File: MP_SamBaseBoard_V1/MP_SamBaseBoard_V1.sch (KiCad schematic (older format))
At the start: 126 parts, among them J1 MA_CONN, J10 P1_CONN, J11 I2C_CONN, J12 I2C_CONN, J13 SAM_SWD, J14 WS2812_EXT, J15 PWR_JACK, J16 USB_B_Micro, J17 BATT_CONN, J2 MB_CONN, J3 Adafruit_Feather_CONN, J4 LOAD_CONN, J5 SPEAKER, J7 SERVO_CONN, J8 P3_CONN, J9 P2_CONN, Q1 DMP3098L, Q2 ALS-PT19-315C/L177/TR8, SW1 RESET, SW2 3v3_PWR_SW, SW3 SW1, SW4 SW2, U1 ESP32-WROOM-32, U10 KXTJ3-1057, U11 IRFHM9331PbF, U13 SST25VF016B-50-4C-S2AF, U2 ATSAMD51J19A-A, U3 74LVC1G125, U4 TPS62135, U5 PAM8301, U6 BQ24075, U7 DRV8833RTY, U8 Sensirion_SHT3x, U9 LD39200PU33R, Y1 Crystal

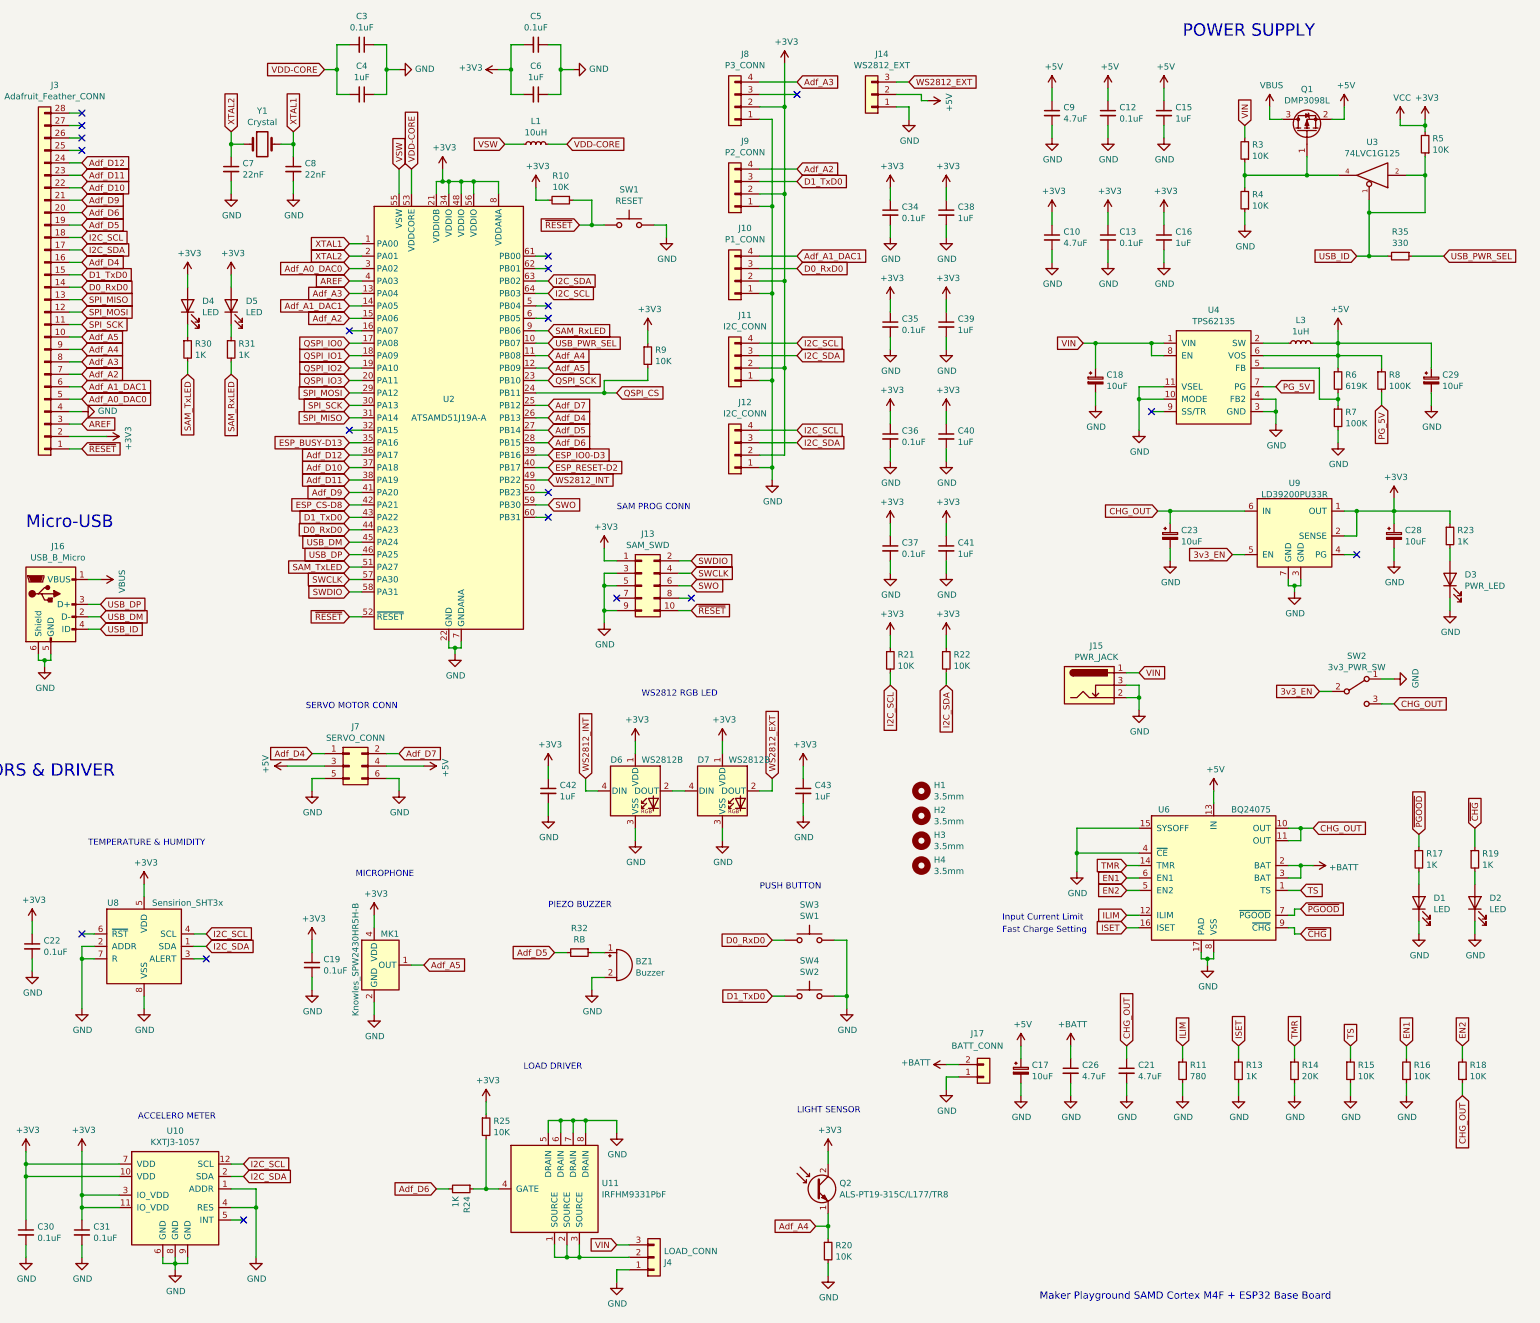
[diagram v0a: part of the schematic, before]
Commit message: update
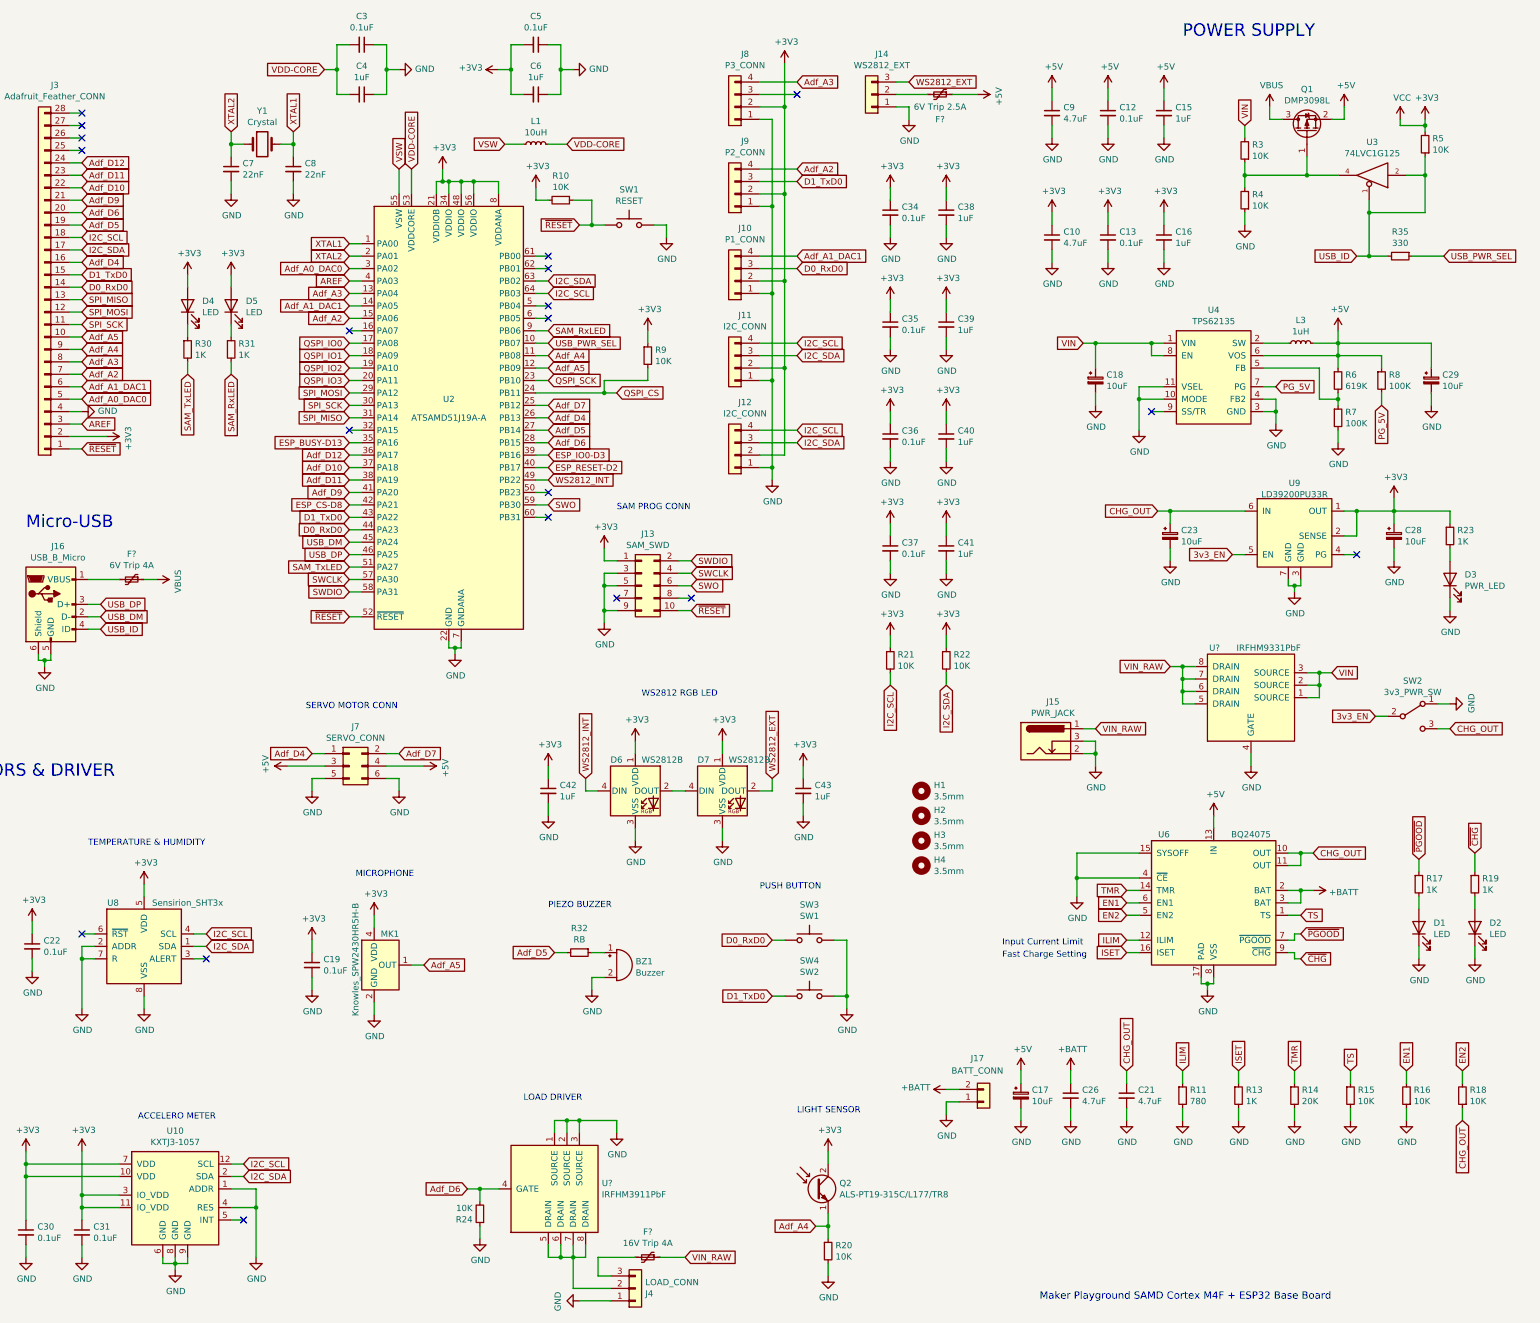
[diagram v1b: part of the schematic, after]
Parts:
- removed R25: 10K, Resistor_SMD:R_0603_1608Metric, symbol Device:R_Small
- removed U11: IRFHM9331PbF, GiraffeTech-IR:PQFN_3x3mm, symbol InGarage_FETs:IRFHM9331PbF
- added F?: 6V Trip 2.5A, Fuse:Fuse_1812_4532Metric, symbol Device:Polyfuse_Small
- added F?: 6V Trip 4A, Fuse:Fuse_1206_3216Metric, symbol Device:Polyfuse_Small
- added F?: 16V Trip 4A, Fuse:Fuse_1812_4532Metric, symbol Device:Polyfuse_Small
- added U?: IRFHM9331PbF, GiraffeTech-IR:PQFN_3x3mm_IRFHM9331TRPbF, symbol InGarage_FETs:IRFHM9331PbF
- added U?: IRFHM3911PbF, GiraffeTech-IR:PQFN_3x3mm_IRFHM3911PbF, symbol InGarage_FETs:IRFHM3911PbF
- R24: value 1K -> 10K
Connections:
- net +5V: now also F?.1; no longer J14.2 (Pin_2)
- net Adf_D6: now also U?.4 (GATE)
- net GND: now also R24.1, U?.1 (SOURCE), U?.2 (SOURCE), U?.3 (SOURCE), U?.4 (GATE)
- net VBUS: now also F?.1; no longer J16.1 (VBUS)
- net VIN: now also U?.1 (SOURCE), U?.2 (SOURCE), U?.3 (SOURCE); no longer J15.1, J4.3 (Pin_3)
- net at J4.2 (Pin_2): now also U?.5 (DRAIN), U?.6 (DRAIN), U?.7 (DRAIN), U?.8 (DRAIN)
- new net: F?.2, J16.1 (VBUS)
- new net: F?.2, J14.2 (Pin_2)
- new net: F?.2, J4.3 (Pin_3)
- new net VIN_RAW: F?.1, J15.1, U?.5 (DRAIN), U?.6 (DRAIN), U?.7 (DRAIN), U?.8 (DRAIN)
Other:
- moved on the sheet: C17, C21, C26, D1, D2, J15, J17, J4, R11, R13, R14, R15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
